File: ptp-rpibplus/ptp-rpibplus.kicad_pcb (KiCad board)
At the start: 2 copper layers, 65.5 x 56.6 mm, 9 parts, among them J1 RASPI_B+, J2 MODULE_HEADER, J3 MODULE_HEADER

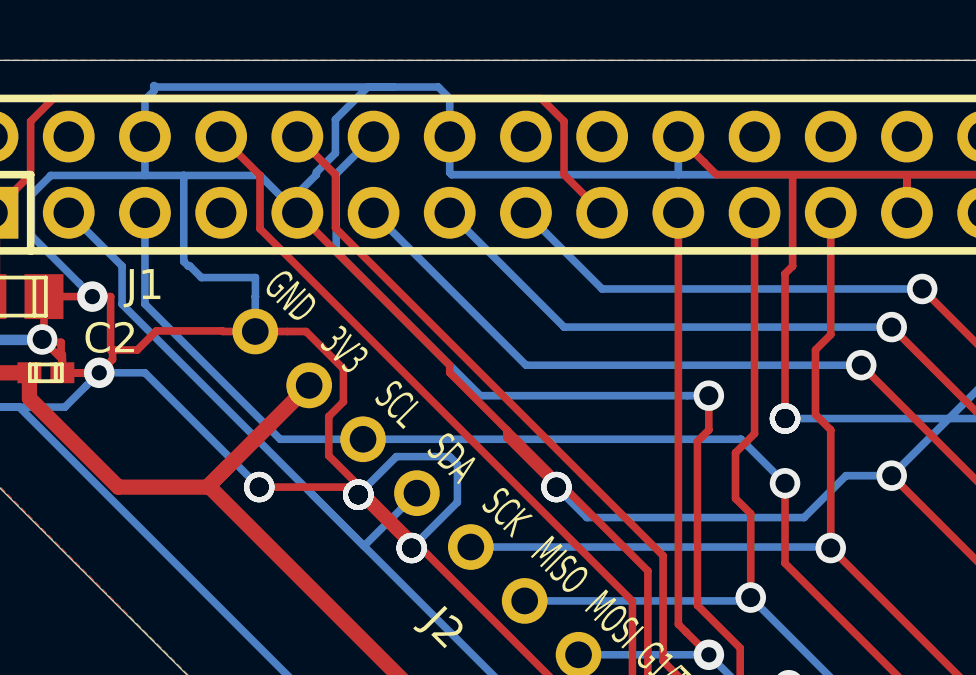
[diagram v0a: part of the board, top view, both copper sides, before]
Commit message: pour tweaks
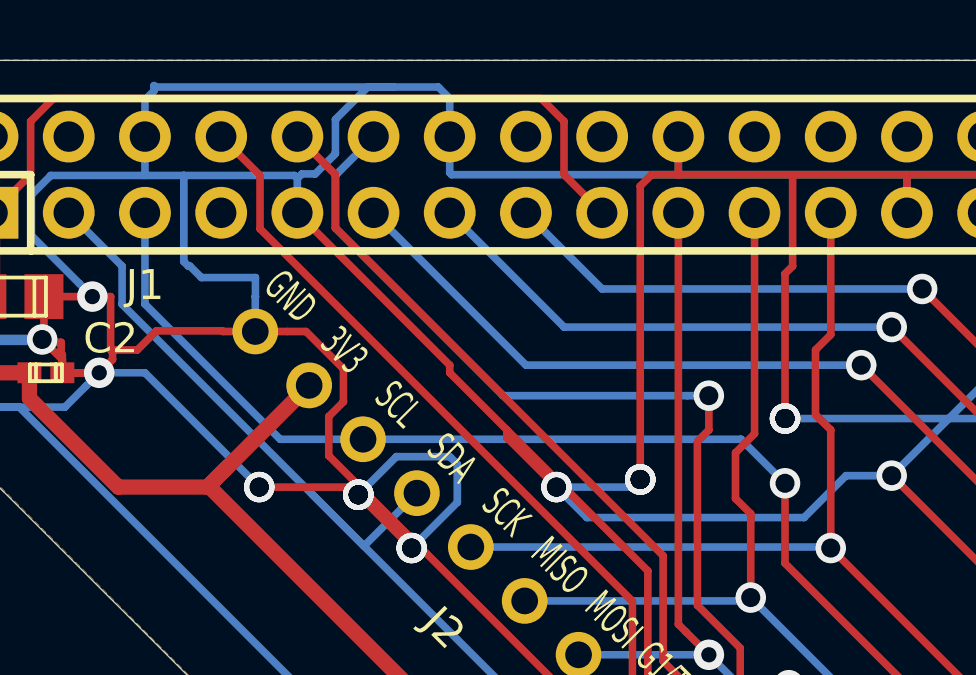
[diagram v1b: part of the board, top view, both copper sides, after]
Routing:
- net GND: track 495.1 -> 509.7 mm, vias 32 -> 36
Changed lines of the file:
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@@
     (thickness 1.6)
     (drawings 84)
-    (tracks 312)
+    (tracks 323)
     (zones 0)
     (modules 9)
@@
   (segment (start 102.65664 84.09686) (end 102.6795 84.074) (width 0.508) (layer F.Cu) (net 1))
   (segment (start 113.424021 87.033421) (end 110.706221 89.751221) (width 0.508) (layer F.Cu) (net 1))
+  (via (at 124.46 90.17) (size 1.016) (drill 0.635) (layers F.Cu B.Cu) (net 2))
+  (segment (start 124.46 90.17) (end 124.46 80.391) (width 0.254) (layer F.Cu) (net 2))
+  (segment (start 124.46 80.391) (end 124.841 80.01) (width 0.254) (layer F.Cu) (net 2))
+  (segment (start 124.841 80.01) (end 125.73 80.01) (width 0.254) (layer F.Cu) (net 2))
+  (via (at 124.46 90.17) (size 1.016) (drill 0.635) (layers F.Cu B.Cu) (net 2))
+  (via (at 124.46 90.17) (size 1.016) (drill 0.635) (layers F.Cu B.Cu) (net 2))
+  (segment (start 121.666 90.424) (end 124.206 90.424) (width 0.254) (layer B.Cu) (net 2))
+  (via (at 124.46 90.17) (size 1.016) (drill 0.635) (layers F.Cu B.Cu) (net 2))
+  (segment (start 124.206 90.424) (end 124.46 90.17) (width 0.254) (layer B.Cu) (net 2))
+  (segment (start 113.03 80.137) (end 112.928399 80.035399) (width 0.254) (layer B.Cu) (net 2))
+  (segment (start 112.928399 80.035399) (end 109.245399 80.035399) (width 0.254) (layer B.Cu) (net 2))
+  (segment (start 114.274601 79.337409) (end 114.274601 79.316965) (width 0.254) (layer B.Cu) (net 2))
+  (segment (start 115.37899 77.089) (end 116.235198 77.089) (width 0.254) (layer B.Cu) (net 2))
+  (segment (start 113.03 81.28) (end 113.03 80.137) (width 0.254) (layer B.Cu) (net 2))
+  (segment (start 114.274601 79.316965) (end 114.3 79.291566) (width 0.254) (layer B.Cu) (net 2))
+  (segment (start 113.03 80.137) (end 113.182399 79.984601) (width 0.254) (layer B.Cu) (net 2))
+  (segment (start 113.182399 79.984601) (end 113.627409 79.984601) (width 0.254) (layer B.Cu) (net 2))
+  (segment (start 113.627409 79.984601) (end 114.274601 79.337409) (width 0.254) (layer B.Cu) (net 2))
+  (segment (start 114.3 79.291566) (end 114.3 78.16799) (width 0.254) (layer B.Cu) (net 2))
+  (segment (start 114.3 78.16799) (end 115.37899 77.089) (width 0.254) (layer B.Cu) (net 2))
+  (segment (start 129.53947 80.01) (end 125.73 80.01) (width 0.254) (layer F.Cu) (net 2))
+  (segment (start 125.73 80.01) (end 125.73 78.74) (width 0.254) (layer F.Cu) (net 2))
   (segment (start 105.19664 86.614) (end 105.19664 86.175716) (width 0.254) (layer F.Cu) (net 2))
   (segment (start 105.19664 86.175716) (end 104.524071 85.503147) (width 0.254) (layer F.Cu) (net 2))
@@
   (segment (start 132.842 90.043) (end 131.318 90.043) (width 0.254) (layer B.Cu) (net 2))
   (segment (start 133.35 80.01) (end 129.53947 80.01) (width 0.254) (layer F.Cu) (net 2))
-  (segment (start 129.53947 80.01) (end 127 80.01) (width 0.254) (layer F.Cu) (net 2))
   (segment (start 129.286 83.312) (end 129.53947 83.05853) (width 0.254) (layer F.Cu) (net 2))
   (segment (start 129.53947 83.05853) (end 129.53947 80.01) (width 0.254) (layer F.Cu) (net 2))
@@
   (segment (start 138.43 80.01) (end 138.43 78.74) (width 0.254) (layer B.Cu) (net 2) (status 20))
   (segment (start 133.35 81.28) (end 133.35 80.01) (width 0.254) (layer B.Cu) (net 2) (status 10))
-  (segment (start 111.785399 80.035399) (end 109.245399 80.035399) (width 0.254) (layer B.Cu) (net 2))
-  (segment (start 113.03 81.28) (end 111.785399 80.035399) (width 0.254) (layer B.Cu) (net 2) (status 10))
   (segment (start 109.245399 80.035399) (end 109.245399 82.905601) (width 0.254) (layer B.Cu) (net 2))
   (segment (start 109.245399 82.905601) (end 109.397798 83.058) (width 0.254) (layer B.Cu) (net 2))
@@
   (segment (start 143.476393 80.01) (end 138.474201 80.01) (width 0.254) (layer F.Cu) (net 2))
   (segment (start 143.501792 79.984601) (end 143.476393 80.01) (width 0.254) (layer F.Cu) (net 2))
-  (segment (start 126.580671 79.590671) (end 125.73 78.74) (width 0.254) (layer F.Cu) (net 2))
-  (segment (start 127 80.01) (end 126.580671 79.590671) (width 0.254) (layer F.Cu) (net 2))
   (segment (start 133.35 81.28) (end 133.35 80.01) (width 0.254) (layer F.Cu) (net 2))
   (segment (start 105.19664 86.01075) (end 105.156 85.97011) (width 0.254) (layer F.Cu) (net 2))
@@
   (segment (start 124.71398 96.666727) (end 125.343329 97.296076) (width 0.254) (layer F.Cu) (net 2))
   (segment (start 131.505958 106.807) (end 124.264335 99.565377) (width 0.254) (layer F.Cu) (net 2))
-  (segment (start 113.03 80.645) (end 113.665 80.01) (width 0.254) (layer B.Cu) (net 2))
-  (segment (start 113.03 81.28) (end 113.03 80.645) (width 0.254) (layer B.Cu) (net 2))
-  (segment (start 113.665 79.926566) (end 114.3 79.291566) (width 0.254) (layer B.Cu) (net 2))
-  (segment (start 113.665 80.01) (end 113.665 79.926566) (width 0.254) (layer B.Cu) (net 2))
-  (segment (start 115.37899 77.089) (end 116.235198 77.089) (width 0.254) (layer B.Cu) (net 2))
-  (segment (start 114.3 78.16799) (end 115.37899 77.089) (width 0.254) (layer B.Cu) (net 2))
-  (segment (start 114.3 79.291566) (end 114.3 78.16799) (width 0.254) (layer B.Cu) (net 2))
   (segment (start 116.235198 77.089) (end 117.729 77.089) (width 0.254) (layer B.Cu) (net 2))
   (segment (start 108.301372 77.089) (end 116.235198 77.089) (width 0.254) (layer B.Cu) (net 2))
@@
   (segment (start 111.785399 81.813399) (end 124.200328 94.228328) (width 0.254) (layer F.Cu) (net 8))
   (segment (start 124.200328 94.228328) (end 124.200328 97.809728) (width 0.254) (layer F.Cu) (net 8))
-  (segment (start 125.22199 92.70999) (end 114.3 81.788) (width 0.254) (layer F.Cu) (net 9))
-  (segment (start 114.3 80.01) (end 113.893599 79.603599) (width 0.254) (layer F.Cu) (net 9))
   (segment (start 125.996379 99.605779) (end 125.996379 96.99849) (width 0.254) (layer F.Cu) (net 9))
   (segment (start 125.996379 96.99849) (end 125.22199 96.224101) (width 0.254) (layer F.Cu) (net 9))
+  (segment (start 125.22199 96.224101) (end 125.22199 92.70999) (width 0.254) (layer F.Cu) (net 9))
+  (segment (start 125.22199 92.70999) (end 114.3 81.788) (width 0.254) (layer F.Cu) (net 9))
+  (segment (start 114.3 81.788) (end 114.3 80.01) (width 0.254) (layer F.Cu) (net 9))
+  (segment (start 114.3 80.01) (end 113.893599 79.603599) (width 0.254) (layer F.Cu) (net 9))
   (segment (start 113.893599 79.603599) (end 113.03 78.74) (width 0.254) (layer F.Cu) (net 9))
-  (segment (start 125.22199 96.224101) (end 125.22199 92.70999) (width 0.254) (layer F.Cu) (net 9))
-  (segment (start 114.3 81.788) (end 114.3 80.01) (width 0.254) (layer F.Cu) (net 9))
   (segment (start 120.65 86.36) (end 115.57 81.28) (width 0.254) (layer B.Cu) (net 10) (status 20))
   (segment (start 131.826 86.36) (end 120.65 86.36) (width 0.254) (layer B.Cu) (net 10))
@@
   (segment (start 145.841128 100.375128) (end 145.841128 119.450528) (width 0.254) (layer F.Cu) (net 10) (status 20))
   (segment (start 131.826 86.36) (end 145.841128 100.375128) (width 0.254) (layer F.Cu) (net 10))
+  (segment (start 115.57 78.74) (end 115.57 78.760444) (width 0.254) (layer B.Cu) (net 11))
+  (segment (start 115.57 78.760444) (end 114.3 80.030444) (width 0.254) (layer B.Cu) (net 11))
+  (segment (start 114.3 80.030444) (end 114.3 81.788) (width 0.254) (layer B.Cu) (net 11))
+  (segment (start 114.3 81.788) (end 119.888 87.376) (width 0.254) (layer B.Cu) (net 11))
+  (segment (start 119.888 87.376) (end 126.02758 87.376) (width 0.254) (layer B.Cu) (net 11))
+  (segment (start 126.02758 87.376) (end 126.746 87.376) (width 0.254) (layer B.Cu) (net 11))
   (segment (start 127.792431 101.401831) (end 127.792431 95.788431) (width 0.254) (layer F.Cu) (net 11))
   (segment (start 127.792431 95.788431) (end 126.365 94.361) (width 0.254) (layer F.Cu) (net 11))
@@
   (segment (start 126.365 88.9) (end 126.746 88.519) (width 0.254) (layer F.Cu) (net 11))
   (segment (start 126.746 88.519) (end 126.746 87.376) (width 0.254) (layer F.Cu) (net 11))
-  (segment (start 126.02758 87.376) (end 126.746 87.376) (width 0.254) (layer B.Cu) (net 11))
-  (segment (start 114.325399 79.984601) (end 114.325399 82.575399) (width 0.254) (layer B.Cu) (net 11))
-  (segment (start 115.57 78.74) (end 114.325399 79.984601) (width 0.254) (layer B.Cu) (net 11))
-  (segment (start 119.126 87.376) (end 126.02758 87.376) (width 0.254) (layer B.Cu) (net 11))
-  (segment (start 114.325399 82.575399) (end 119.126 87.376) (width 0.254) (layer B.Cu) (net 11))
   (via (at 126.746 87.376) (size 1.016) (drill 0.635) (layers F.Cu B.Cu) (net 11))
   (segment (start 121.92 85.09) (end 118.11 81.28) (width 0.254) (layer B.Cu) (net 12) (status 20))
@@
       )
     )
+  )
+  (zone (net 0) (net_name "") (layer B.Cu) (hatch edge 0.508)
+    (connect_pads (clearance 0.254))
+    (min_thickness 0.254)
+    (keepout (tracks not_allowed) (vias not_allowed) (copperpour not_allowed))
+    (fill yes (arc_segments 16) (thermal_gap 0.254) (thermal_bridge_width 0.508))
+    (polygon
+      (pts
+        (xy 116.586 81.153) (xy 121.412 81.153) (xy 121.412 81.661) (xy 116.586 81.661)
+      )
+    )
